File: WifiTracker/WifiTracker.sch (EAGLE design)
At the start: 29 parts, among them IC1 TS1117CP33-R0, Q1 BSS123, Q2 BSS123, Y1 16MHz

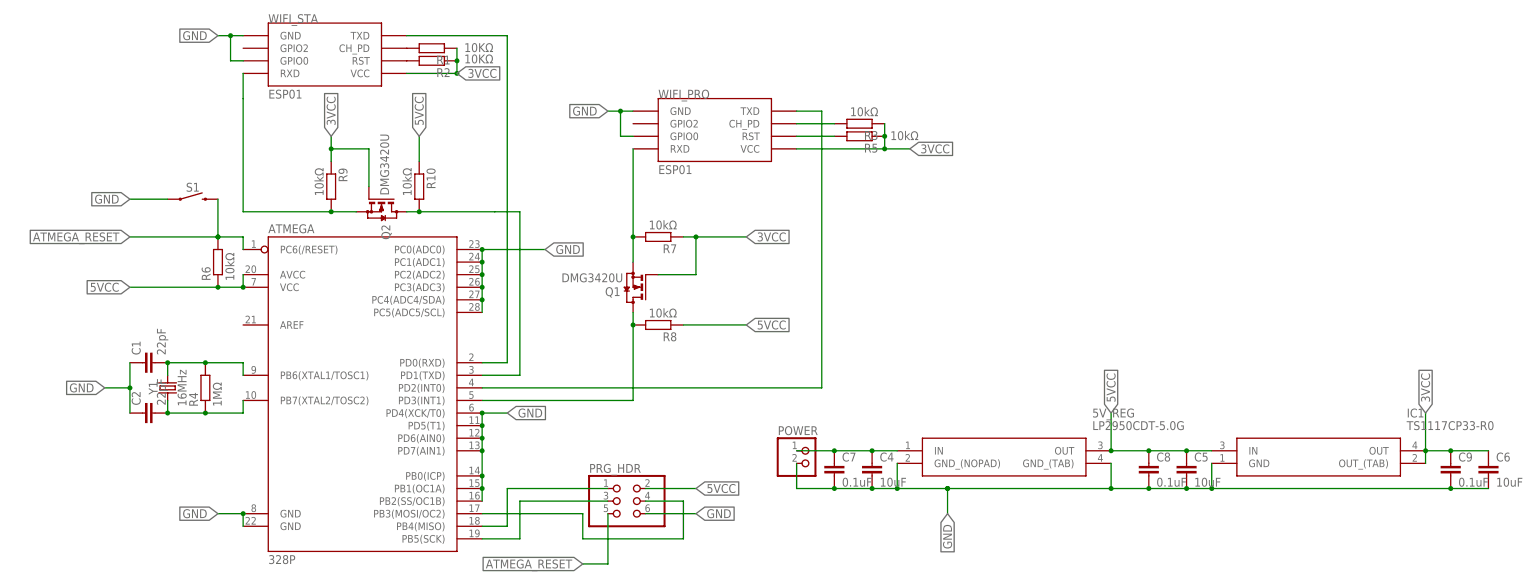
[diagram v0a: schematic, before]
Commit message: Prepare to print
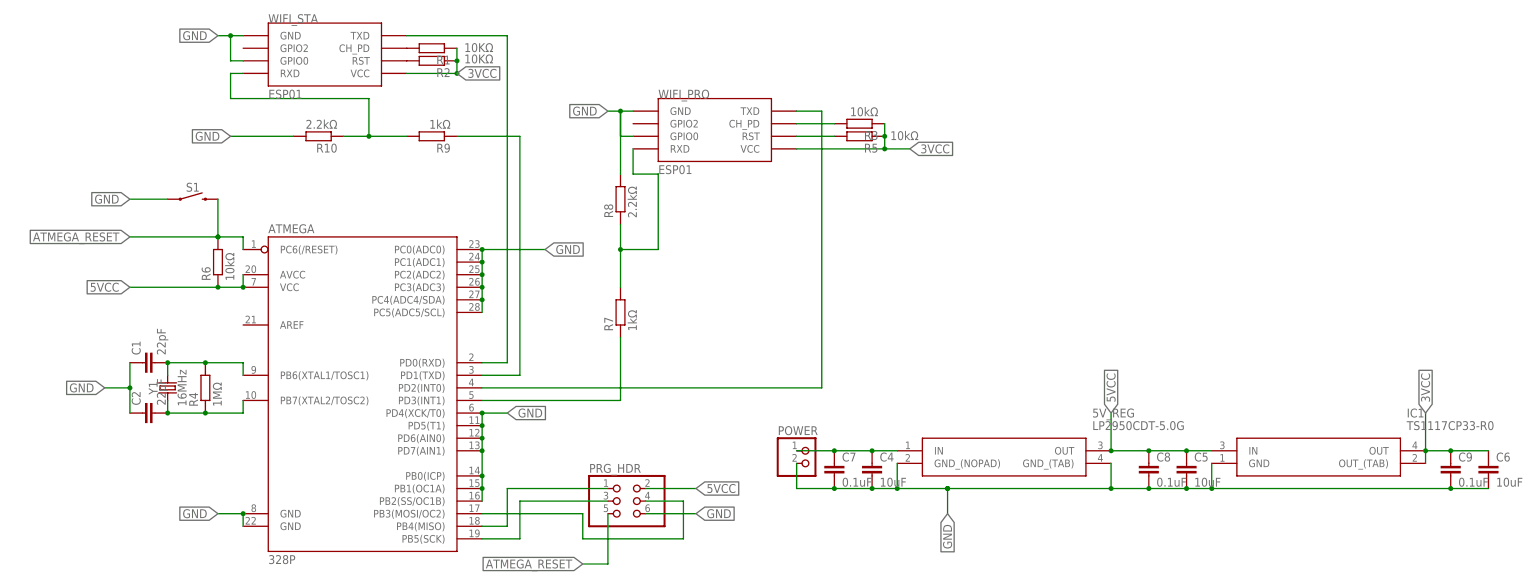
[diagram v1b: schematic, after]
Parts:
- removed Q1, Q2: BSS123, transistor-small-signal:BSS123
- R10, R8: value 10kΩ -> 2.2kΩ
- R7, R9: value 10kΩ -> 1kΩ
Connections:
- removed net N$1: WIFI_PRO.TXD
- removed net N$2: WIFI_STA.RXD
- removed net N$3: Q1.S, R7.2, WIFI_PRO.RXD
- removed net N$4: Q2.S, R9.2
- removed net PRO_RXD1: Q2.D, R10.2
- new net AT_STXD: ATMEGA.PD3(INT1), R7.1
- new net AT_TXD: ATMEGA.PD1(TXD), R9.1
- net 3VCC: no longer Q1.G, Q2.G, R7.1, R9.1
- net 5VCC: no longer R10.1, R8.1
- net GND: now also R10.2, R8.2
- net PRO_RXD: now also R7.2, R8.1, WIFI_PRO.RXD; no longer ATMEGA.PD3(INT1), Q1.D, R8.2
- net PRO_TXD: now also WIFI_PRO.TXD
- net STA_RXD: now also R10.1, R9.2, WIFI_STA.RXD; no longer ATMEGA.PD1(TXD)
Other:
- note removed: "DMG3420U"
- moved on the sheet: R10, R7, R8, R9
